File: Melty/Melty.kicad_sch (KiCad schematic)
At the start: 35 parts, among them J1 ESC signal, J2 ESC Power, J3 ESC Power, J4 Power In, J5 Switch, Q1 BSS138, Q2 BSS138, Q3 BSS138, U1 XIAO-ESP32-C3-DIP, U2 H3LIS331DLTR, U3 TLV76150DCY, U4 ELRS, U5 TSSP58038

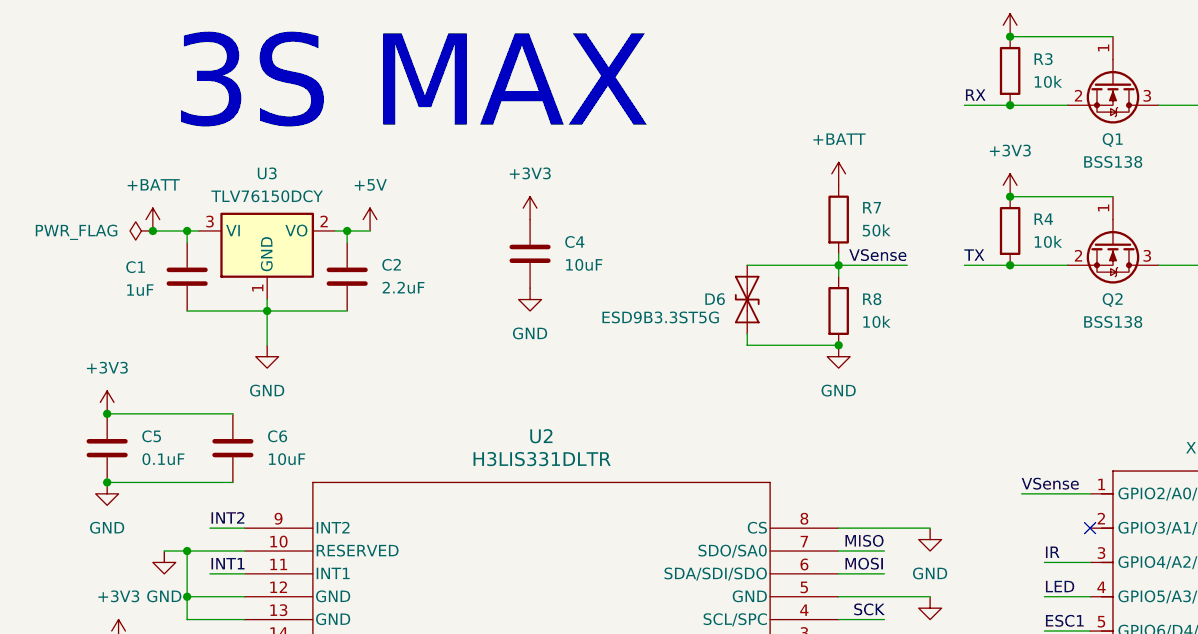
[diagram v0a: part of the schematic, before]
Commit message: crsf reading
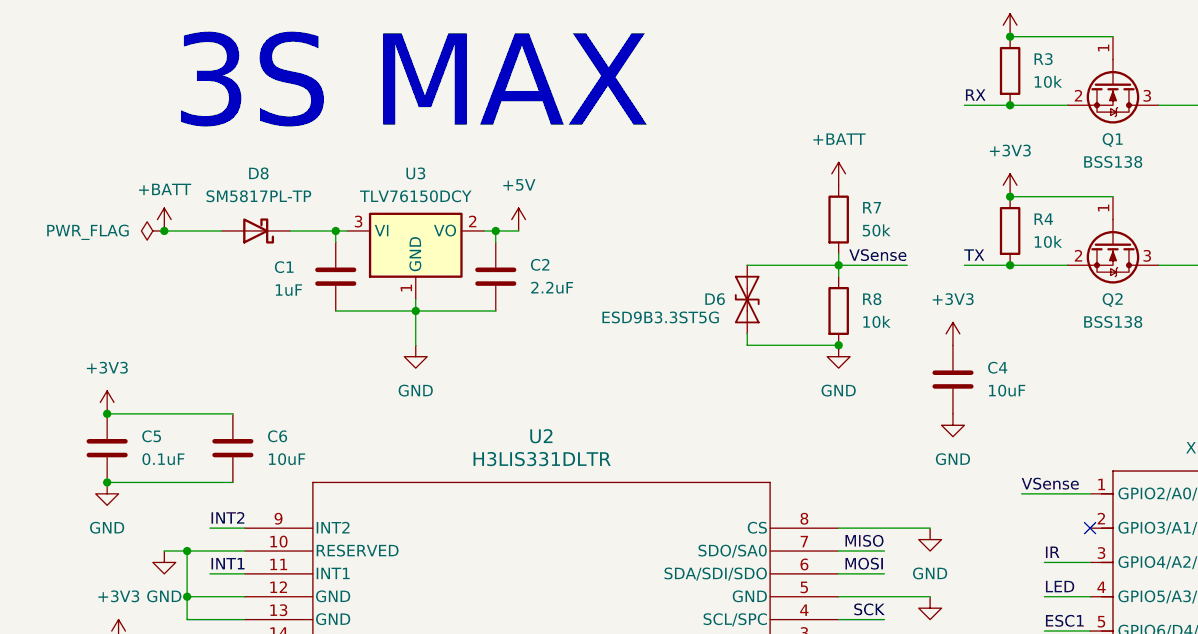
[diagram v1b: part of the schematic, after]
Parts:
- added D8: SM5817PL-TP, symbol Device:D_Schottky
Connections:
- net +BATT: now also D8.2 (A); no longer C1.1, U3.3 (VI)
- new net: C1.1, D8.1 (K), U3.3 (VI)
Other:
- moved on the sheet: C1, C2, C4, U3
